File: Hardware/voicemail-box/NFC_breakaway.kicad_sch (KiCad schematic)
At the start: 22 parts, among them U501 ST25R3916B, Y501 27.12Mhz

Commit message: HW Layout progress todo: + Antenna + Audio Jacks + Planes (Supply only)
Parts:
- C501, C502, C503, C504, C505, C506, C507, C508, C509, C510, C511, C512, C513, C514, C515, C516, C517, C518, C519: footprint Capacitor_SMD:C_0201_0603Metric_Pad0.64x0.40mm_HandSolder -> Capacitor_SMD:C_0603_1608Metric_Pad1.08x0.95mm_HandSolder
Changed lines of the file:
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@@
 			)
 		)
-		(property "Footprint" "Capacitor_SMD:C_0201_0603Metric_Pad0.64x0.40mm_HandSolder"
+		(property "Footprint" "Capacitor_SMD:C_0603_1608Metric_Pad1.08x0.95mm_HandSolder"
 			(at 27.6352 149.86 0)
 			(effects
@@
 			)
 		)
-		(property "Footprint" "Capacitor_SMD:C_0201_0603Metric_Pad0.64x0.40mm_HandSolder"
+		(property "Footprint" "Capacitor_SMD:C_0603_1608Metric_Pad1.08x0.95mm_HandSolder"
 			(at 50.4952 149.86 0)
 			(effects
@@
 			)
 		)
-		(property "Footprint" "Capacitor_SMD:C_0201_0603Metric_Pad0.64x0.40mm_HandSolder"
+		(property "Footprint" "Capacitor_SMD:C_0603_1608Metric_Pad1.08x0.95mm_HandSolder"
 			(at 209.2452 143.51 0)
 			(effects
@@
 			)
 		)
-		(property "Footprint" "Capacitor_SMD:C_0201_0603Metric_Pad0.64x0.40mm_HandSolder"
+		(property "Footprint" "Capacitor_SMD:C_0603_1608Metric_Pad1.08x0.95mm_HandSolder"
 			(at 113.9952 143.51 0)
 			(effects
@@
 			)
 		)
-		(property "Footprint" "Capacitor_SMD:C_0201_0603Metric_Pad0.64x0.40mm_HandSolder"
+		(property "Footprint" "Capacitor_SMD:C_0603_1608Metric_Pad1.08x0.95mm_HandSolder"
 			(at 93.6752 143.51 0)
 			(effects
@@
 			)
 		)
-		(property "Footprint" "Capacitor_SMD:C_0201_0603Metric_Pad0.64x0.40mm_HandSolder"
+		(property "Footprint" "Capacitor_SMD:C_0603_1608Metric_Pad1.08x0.95mm_HandSolder"
 			(at 260.0452 143.51 0)
 			(effects
@@
 			)
 		)
-		(property "Footprint" "Capacitor_SMD:C_0201_0603Metric_Pad0.64x0.40mm_HandSolder"
+		(property "Footprint" "Capacitor_SMD:C_0603_1608Metric_Pad1.08x0.95mm_HandSolder"
 			(at 154.6352 143.51 0)
 			(effects
@@
 			)
 		)
-		(property "Footprint" "Capacitor_SMD:C_0201_0603Metric_Pad0.64x0.40mm_HandSolder"
+		(property "Footprint" "Capacitor_SMD:C_0603_1608Metric_Pad1.08x0.95mm_HandSolder"
 			(at 73.3552 143.51 0)
 			(effects
@@
 			)
 		)
-		(property "Footprint" "Capacitor_SMD:C_0201_0603Metric_Pad0.64x0.40mm_HandSolder"
+		(property "Footprint" "Capacitor_SMD:C_0603_1608Metric_Pad1.08x0.95mm_HandSolder"
 			(at 134.3152 143.51 0)
 			(effects
@@
 			)
 		)
-		(property "Footprint" "Capacitor_SMD:C_0201_0603Metric_Pad0.64x0.40mm_HandSolder"
+		(property "Footprint" "Capacitor_SMD:C_0603_1608Metric_Pad1.08x0.95mm_HandSolder"
 			(at 239.7252 143.51 0)
 			(effects
@@
 			)
 		)
-		(property "Footprint" "Capacitor_SMD:C_0201_0603Metric_Pad0.64x0.40mm_HandSolder"
+		(property "Footprint" "Capacitor_SMD:C_0603_1608Metric_Pad1.08x0.95mm_HandSolder"
 			(at 83.5152 143.51 0)
 			(effects
@@
 			)
 		)
-		(property "Footprint" "Capacitor_SMD:C_0201_0603Metric_Pad0.64x0.40mm_HandSolder"
+		(property "Footprint" "Capacitor_SMD:C_0603_1608Metric_Pad1.08x0.95mm_HandSolder"
 			(at 219.4052 143.51 0)
 			(effects
@@
 			)
 		)
-		(property "Footprint" "Capacitor_SMD:C_0201_0603Metric_Pad0.64x0.40mm_HandSolder"
+		(property "Footprint" "Capacitor_SMD:C_0603_1608Metric_Pad1.08x0.95mm_HandSolder"
 			(at 229.5652 143.51 0)
 			(effects
@@
 			)
 		)
-		(property "Footprint" "Capacitor_SMD:C_0201_0603Metric_Pad0.64x0.40mm_HandSolder"
+		(property "Footprint" "Capacitor_SMD:C_0603_1608Metric_Pad1.08x0.95mm_HandSolder"
 			(at 249.8852 143.51 0)
 			(effects
@@
 			)
 		)
-		(property "Footprint" "Capacitor_SMD:C_0201_0603Metric_Pad0.64x0.40mm_HandSolder"
+		(property "Footprint" "Capacitor_SMD:C_0603_1608Metric_Pad1.08x0.95mm_HandSolder"
 			(at 144.4752 143.51 0)
 			(effects
@@
 			)
 		)
-		(property "Footprint" "Capacitor_SMD:C_0201_0603Metric_Pad0.64x0.40mm_HandSolder"
+		(property "Footprint" "Capacitor_SMD:C_0603_1608Metric_Pad1.08x0.95mm_HandSolder"
 			(at 103.8352 143.51 0)
 			(effects
@@
 			)
 		)
-		(property "Footprint" "Capacitor_SMD:C_0201_0603Metric_Pad0.64x0.40mm_HandSolder"
+		(property "Footprint" "Capacitor_SMD:C_0603_1608Metric_Pad1.08x0.95mm_HandSolder"
 			(at 199.0852 143.51 0)
 			(effects
@@
 			)
 		)
-		(property "Footprint" "Capacitor_SMD:C_0201_0603Metric_Pad0.64x0.40mm_HandSolder"
+		(property "Footprint" "Capacitor_SMD:C_0603_1608Metric_Pad1.08x0.95mm_HandSolder"
 			(at 270.2052 143.51 0)
 			(effects
@@
 			)
 		)
-		(property "Footprint" "Capacitor_SMD:C_0201_0603Metric_Pad0.64x0.40mm_HandSolder"
+		(property "Footprint" "Capacitor_SMD:C_0603_1608Metric_Pad1.08x0.95mm_HandSolder"
 			(at 124.1552 143.51 0)
 			(effects

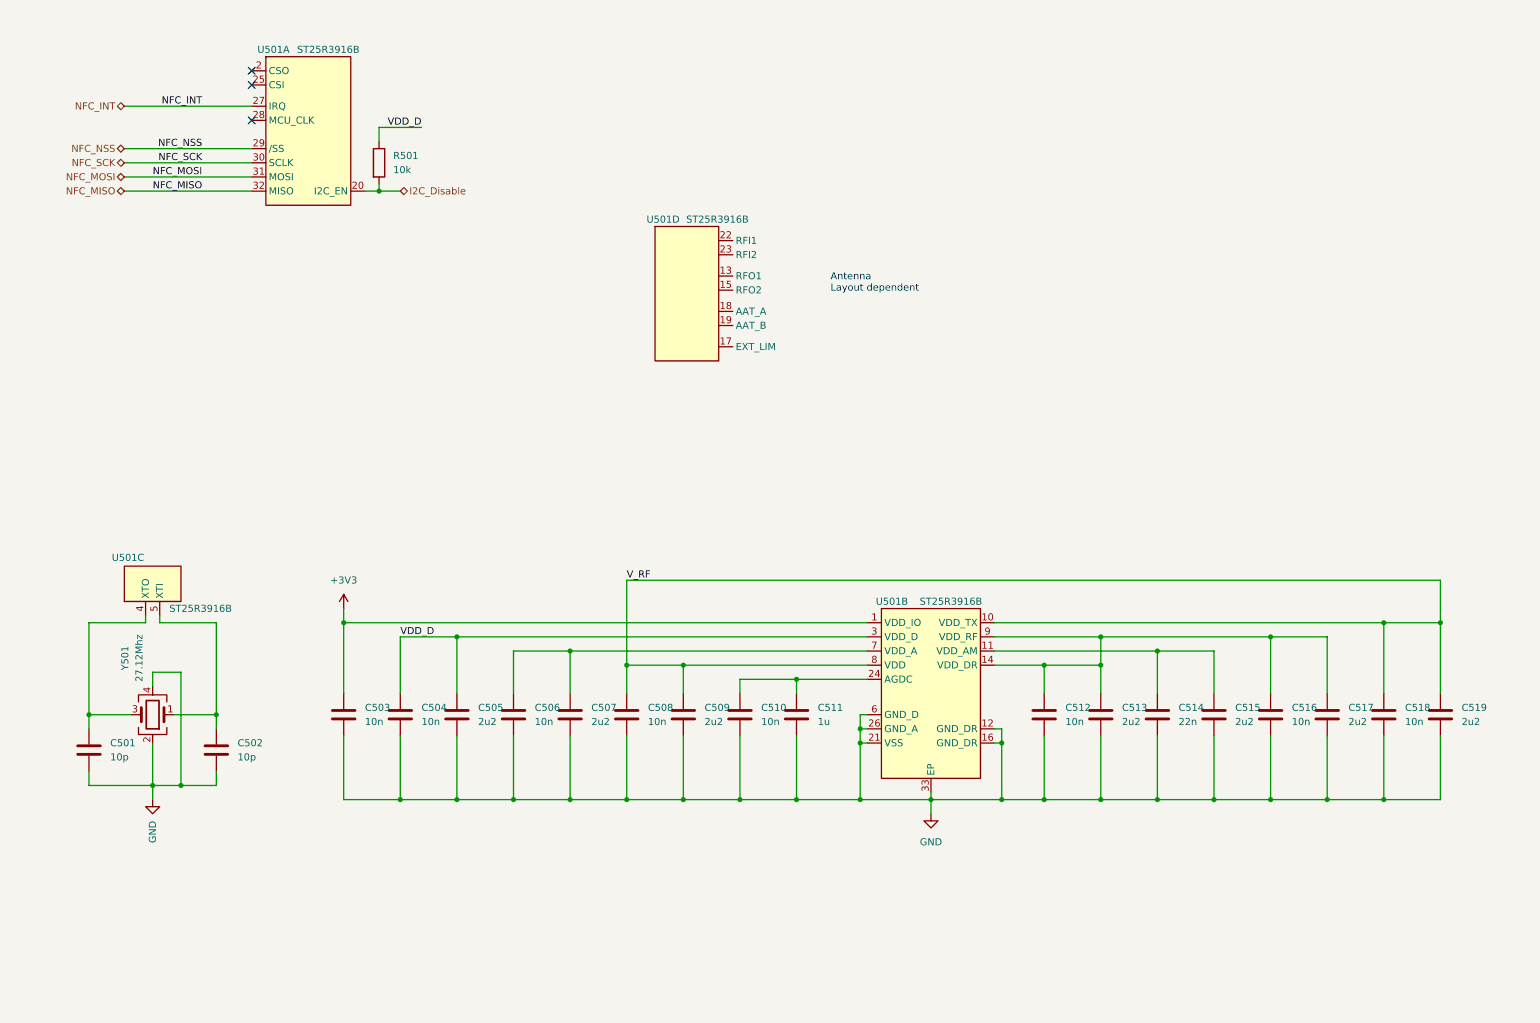
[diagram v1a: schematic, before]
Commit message: schema review
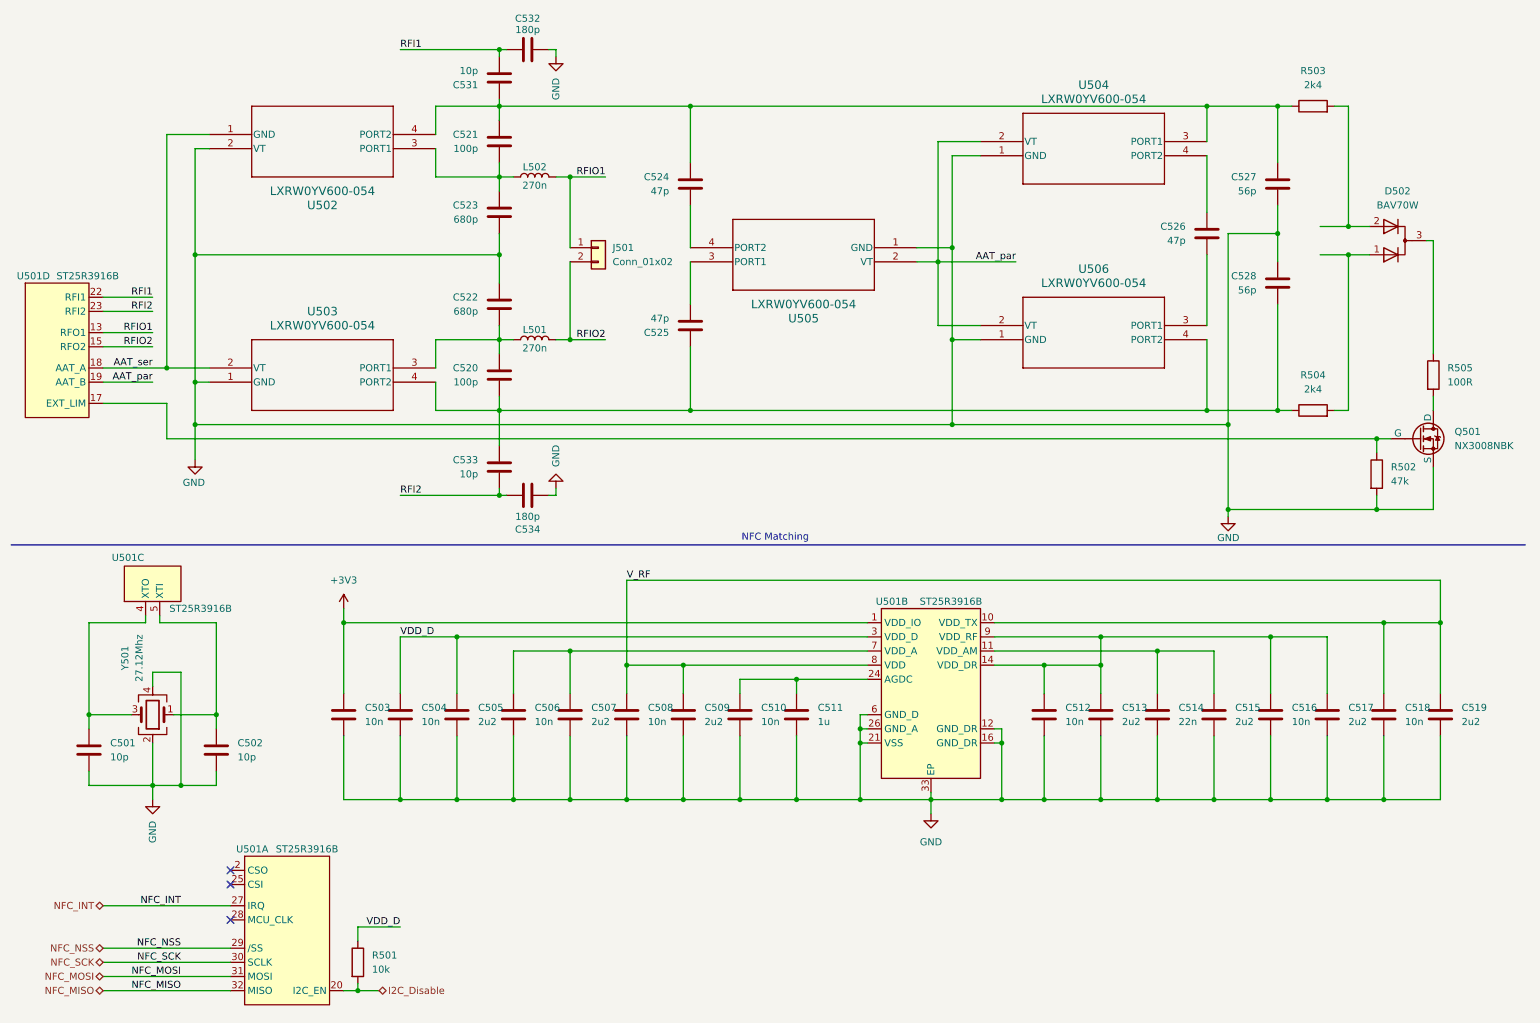
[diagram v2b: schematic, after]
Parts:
- added C520, C521: 100p, Capacitor_SMD:C_0603_1608Metric_Pad1.08x0.95mm_HandSolder, symbol Device:C
- added C522, C523: 680p, Capacitor_SMD:C_0603_1608Metric_Pad1.08x0.95mm_HandSolder, symbol Device:C
- added C524, C525, C526: 47p, Capacitor_SMD:C_0603_1608Metric_Pad1.08x0.95mm_HandSolder, symbol Device:C
- added C527, C528: 56p, Capacitor_SMD:C_0603_1608Metric_Pad1.08x0.95mm_HandSolder, symbol Device:C
- added C531, C533: 10p, Capacitor_SMD:C_0603_1608Metric_Pad1.08x0.95mm_HandSolder, symbol Device:C
- added C532, C534: 180p, Capacitor_SMD:C_0603_1608Metric_Pad1.08x0.95mm_HandSolder, symbol Device:C
- added D502: BAV70W, Package_TO_SOT_SMD:SOT-23-3, symbol Device:D_Dual_CommonCathode_AAK_Parallel
- added J501: Conn_01x02, Connector_PinHeader_1.27mm:PinHeader_1x02_P1.27mm_Vertical, symbol Connector_Generic:Conn_01x02
- added L501, L502: 270n, symbol Device:L
- added Q501: NX3008NBK, Package_TO_SOT_SMD:SOT-23-3, symbol Simulation_SPICE:NMOS
- added R502: 47k, Resistor_SMD:R_0805_2012Metric_Pad1.20x1.40mm_HandSolder, symbol Device:R
- added R503, R504: 2k4, Resistor_SMD:R_0805_2012Metric_Pad1.20x1.40mm_HandSolder, symbol Device:R
- added R505: 100R, Resistor_SMD:R_0805_2012Metric_Pad1.20x1.40mm_HandSolder, symbol Device:R
- added U502, U503, U504, U505, U506: LXRW0YV600-054, LXRW0_MUR, symbol additial parts:LXRW0YV600-054
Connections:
- net GND: now also C522.1, C523.2, C527.2, C528.1, C532.1, C534.1, Q501.3 (S), R502.2, U502.2 (VT), U503.1 (GND), U504.1 (GND), U505.1 (GND), U506.1 (GND)
- net RFIO1: now reaches U501.13 (RFO1)
- net RFIO1: now also J501.1 (Pin_1), L502.2
- net RFIO2: now reaches U501.15 (RFO2)
- net RFIO2: now also J501.2 (Pin_2), L501.2
- net at U501.17 (EXT_LIM): now also Q501.2 (G), R502.1
- net AAT_ser: now reaches U501.18 (AAT_A)
- net AAT_ser: now also U502.1 (GND), U503.2 (VT)
- net AAT_par: now reaches U501.19 (AAT_B)
- net AAT_par: now also U504.2 (VT), U505.2 (VT), U506.2 (VT)
- net RFI1: now reaches U501.22 (RFI1)
- net RFI1: now also C531.2, C532.2
- net RFI2: now reaches U501.23 (RFI2)
- net RFI2: now also C533.2, C534.2
- new net: C520.2, C525.1, C528.2, C533.1, R504.1, U503.4 (PORT2), U506.4 (PORT2)
- new net: C525.2, U505.3 (PORT1)
- new net: D502.3 (K), R505.1
- new net: Q501.1 (D), R505.2
- new net: C520.1, C522.2, L501.1, U503.3 (PORT1)
- new net: C521.1, C524.1, C527.1, C531.1, R503.1, U502.4 (PORT2), U504.3 (PORT1)
- new net: C526.2, U506.3 (PORT1)
- new net: C521.2, C523.1, L502.1, U502.3 (PORT1)
- new net: D502.2 (A), R503.2
- new net: D502.1 (A), R504.2
- new net: C524.2, U505.4 (PORT2)
- new net: C526.1, U504.4 (PORT2)
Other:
- note added: "NFC Matching"
- note removed: "Antenna Layout dependent"
- moved on the sheet: R501, U501A, U501D

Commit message: ~layout
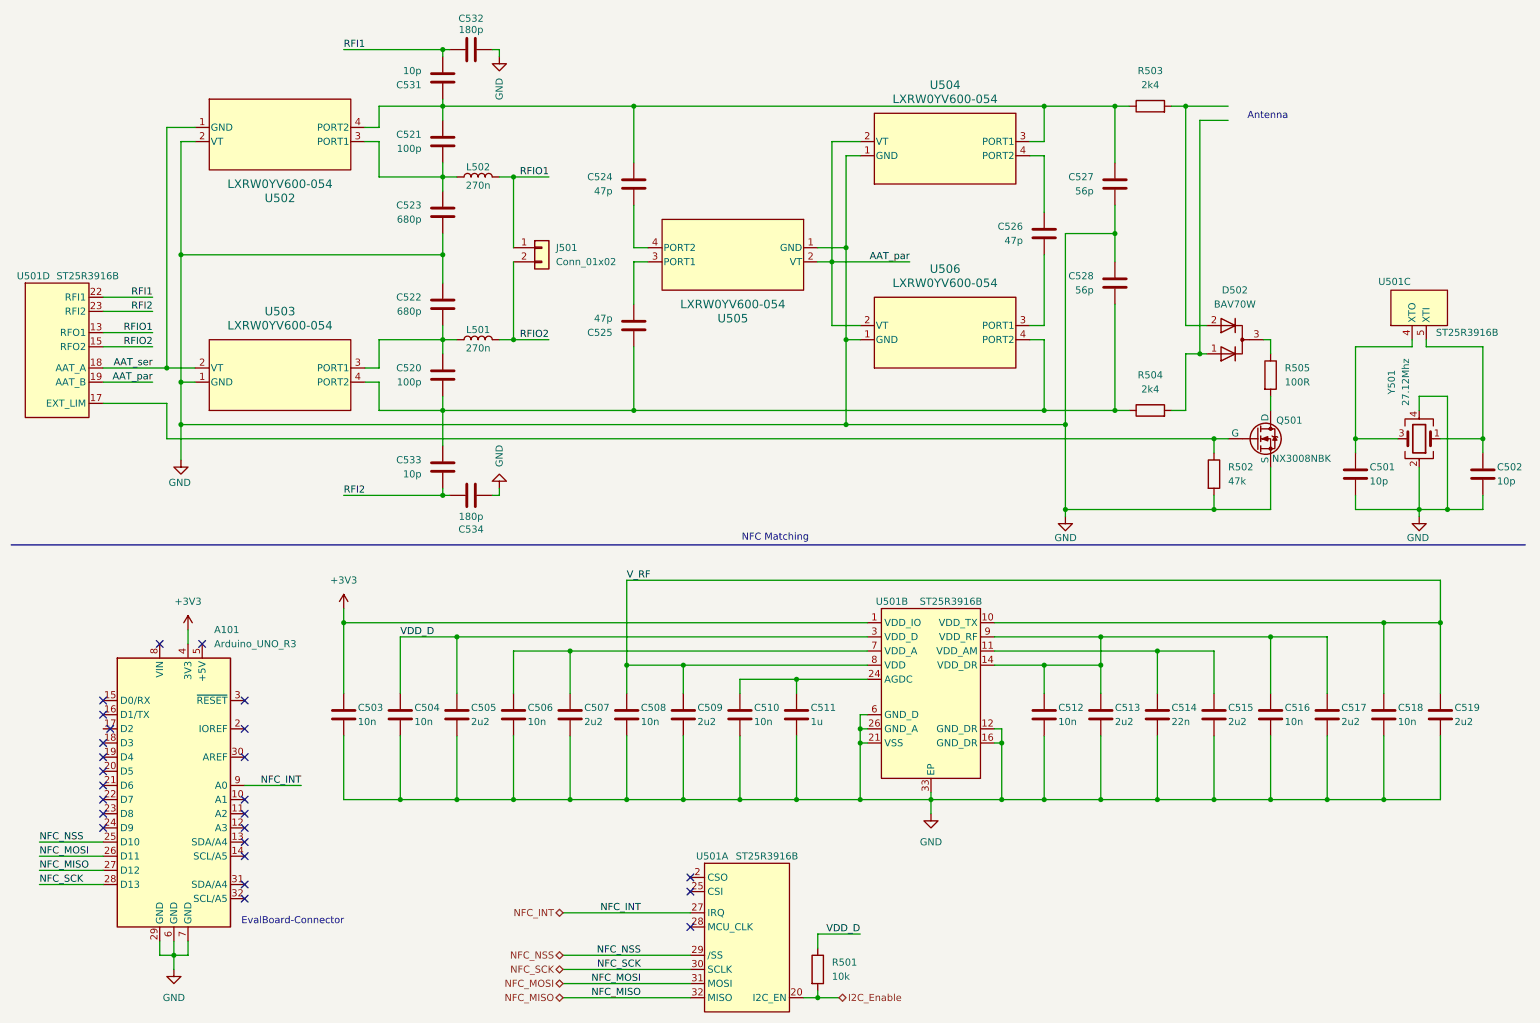
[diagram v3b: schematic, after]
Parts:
- added A101: Arduino_UNO_R3, Module:Arduino_UNO_R3, symbol MCU_Module:Arduino_UNO_R3
- L501, L502: footprint (none) -> Inductor_SMD:L_0603_1608Metric_Pad1.05x0.95mm_HandSolder
- U502, U503, U504, U505, U506: footprint LXRW0_MUR -> additional parts:LXRW0_MUR-M
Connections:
- net +3V3: now also A101.4 (3V3)
- net GND: now also A101.29 (GND), A101.6 (GND), A101.7 (GND)
- net NFC_INT: now also A101.9 (A0)
- net NFC_MISO: now also A101.27 (D12)
- net NFC_MOSI: now also A101.26 (D11)
- net NFC_NSS: now also A101.25 (D10)
- net NFC_SCK: now also A101.28 (D13)
- net I2C_Disable renamed I2C_Enable
- no-connect marks 3 -> 25
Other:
- note added: "Antenna"
- note added: "EvalBoard-Connector"
- moved on the sheet: C501, C502, C520, C521, C522, C523, C524, C525, C526, C527, C528, C531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
